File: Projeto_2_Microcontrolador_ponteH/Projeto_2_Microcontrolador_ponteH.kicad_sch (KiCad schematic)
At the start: 0 parts

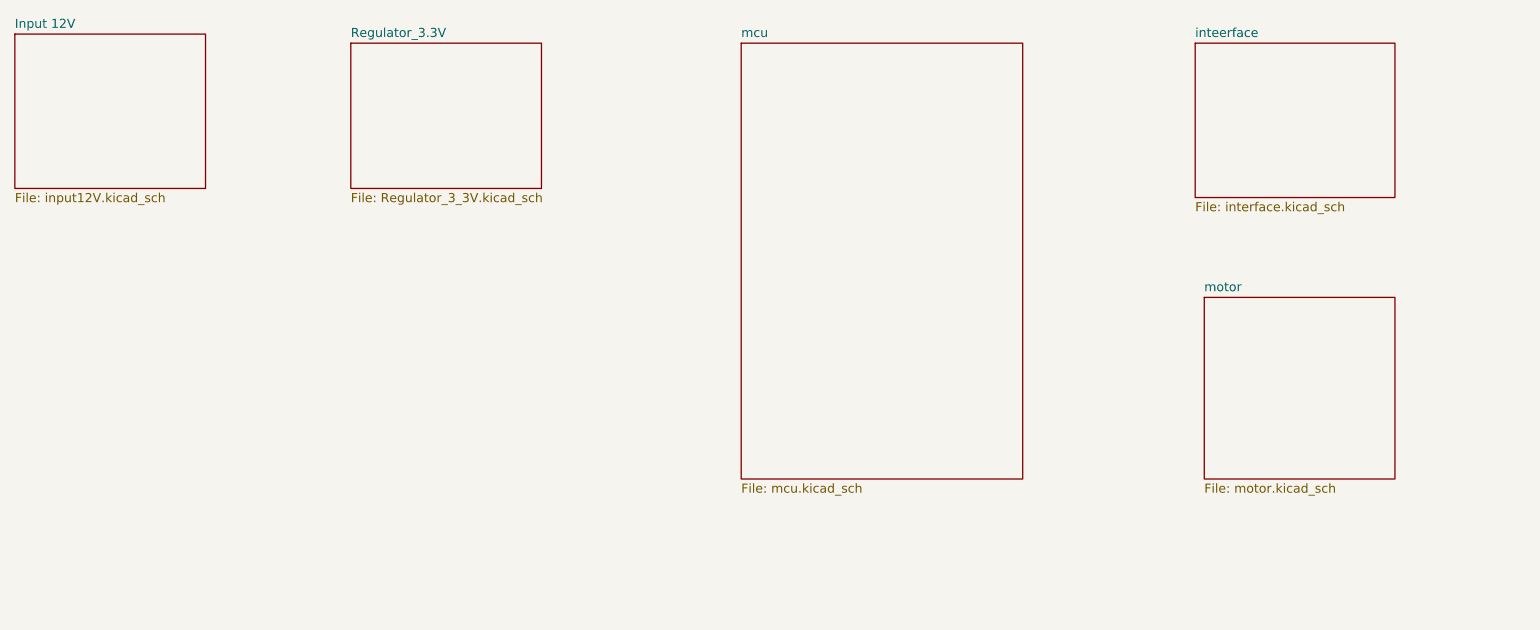
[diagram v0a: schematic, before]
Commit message: Atualização
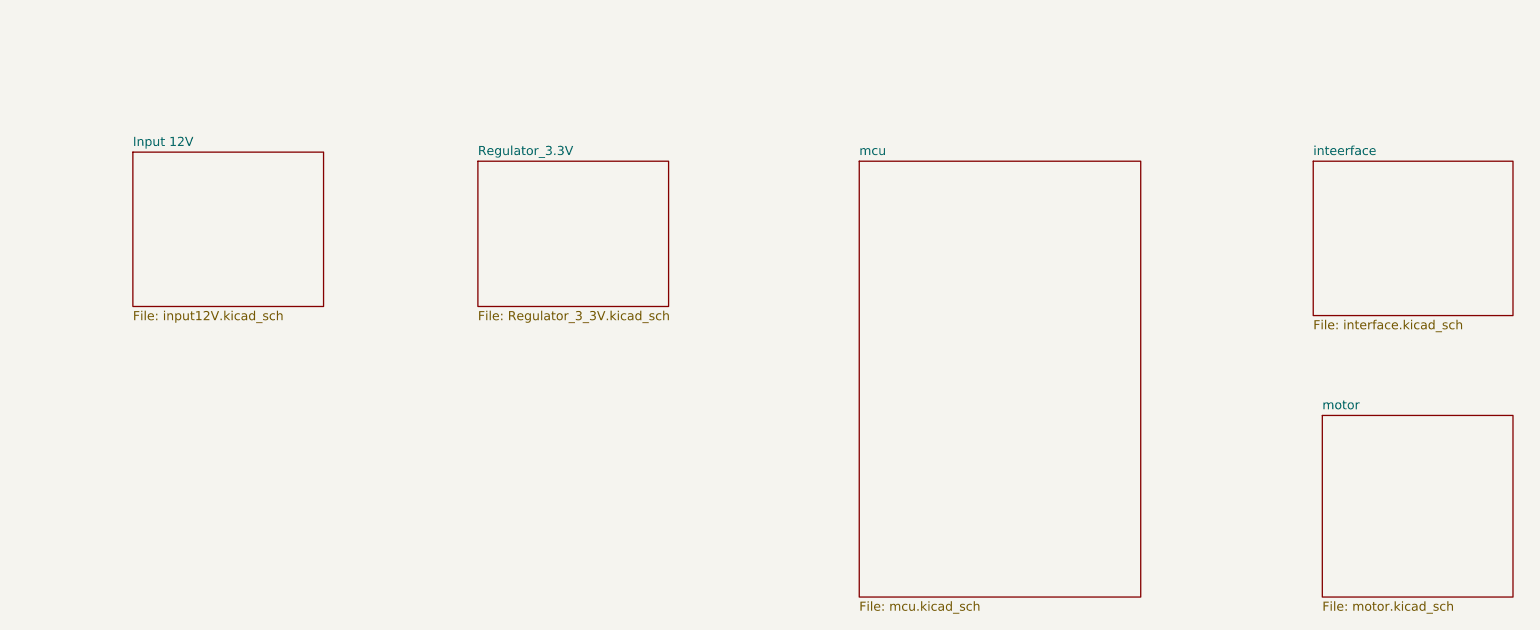
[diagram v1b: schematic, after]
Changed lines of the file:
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@@
 	(paper "A4")
 	(sheet
-		(at 194.31 83.82)
+		(at 210.82 100.33)
 		(size 26.67 25.4)
 		(exclude_from_sim no)
@@
 		)
 		(property "Sheetname" "motor"
-			(at 194.31 83.1084 0)
+			(at 210.82 99.6184 0)
 			(show_name no)
 			(do_not_autoplace no)
@@
 		)
 		(property "Sheetfile" "motor.kicad_sch"
-			(at 194.31 109.8046 0)
+			(at 210.82 126.3146 0)
 			(show_name no)
 			(do_not_autoplace no)
@@
 	)
 	(sheet
-		(at 74.93 48.26)
+		(at 92.71 64.77)
 		(size 26.67 20.32)
 		(exclude_from_sim no)
@@
 		)
 		(property "Sheetname" "Regulator_3.3V"
-			(at 74.93 47.5484 0)
+			(at 92.71 64.0584 0)
 			(show_name no)
 			(do_not_autoplace no)
@@
 		)
 		(property "Sheetfile" "Regulator_3_3V.kicad_sch"
-			(at 74.93 69.1646 0)
+			(at 92.71 85.6746 0)
 			(show_name no)
 			(do_not_autoplace no)
@@
 	)
 	(sheet
-		(at 129.54 48.26)
+		(at 146.05 64.77)
 		(size 39.37 60.96)
 		(exclude_from_sim no)
@@
 		)
 		(property "Sheetname" "mcu"
-			(at 129.54 47.5484 0)
+			(at 146.05 64.0584 0)
 			(show_name no)
 			(do_not_autoplace no)
@@
 		)
 		(property "Sheetfile" "mcu.kicad_sch"
-			(at 129.54 109.8046 0)
+			(at 146.05 126.3146 0)
 			(show_name no)
 			(do_not_autoplace no)
@@
 	)
 	(sheet
-		(at 193.04 48.26)
+		(at 209.55 64.77)
 		(size 27.94 21.59)
 		(exclude_from_sim no)
@@
 		)
 		(property "Sheetname" "inteerface"
-			(at 193.04 47.5484 0)
+			(at 209.55 64.0584 0)
 			(show_name no)
 			(do_not_autoplace no)
@@
 		)
 		(property "Sheetfile" "interface.kicad_sch"
-			(at 193.04 70.4346 0)
+			(at 209.55 86.9446 0)
 			(show_name no)
 			(do_not_autoplace no)
@@
 	)
 	(sheet
-		(at 27.94 46.99)
+		(at 44.45 63.5)
 		(size 26.67 21.59)
 		(exclude_from_sim no)
@@
 		)
 		(property "Sheetname" "Input 12V"
-			(at 27.94 46.2784 0)
+			(at 44.45 62.7884 0)
 			(show_name no)
 			(do_not_autoplace no)
@@
 		)
 		(property "Sheetfile" "input12V.kicad_sch"
-			(at 27.94 69.1646 0)
-			(show_name no)
-			(do_not_autoplace no)
+			(at 44.45 85.6746 0)
+			(show_name no)
+			(do_not_autoplace no)
